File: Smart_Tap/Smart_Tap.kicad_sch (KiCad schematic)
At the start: 30 parts, among them IC1 TCRT5000L, IC2 TCRT5000L, IC3 PIC16C745-I_SO, J1 USB_B_Micro, J2 Conn_01x02_Female, J3 USB_B_Micro, M1 Motor_Servo, Q1 BC547, U1 MCP73831-2-OT, U2 LM393, U3 LM393, U4 DRV8833PW

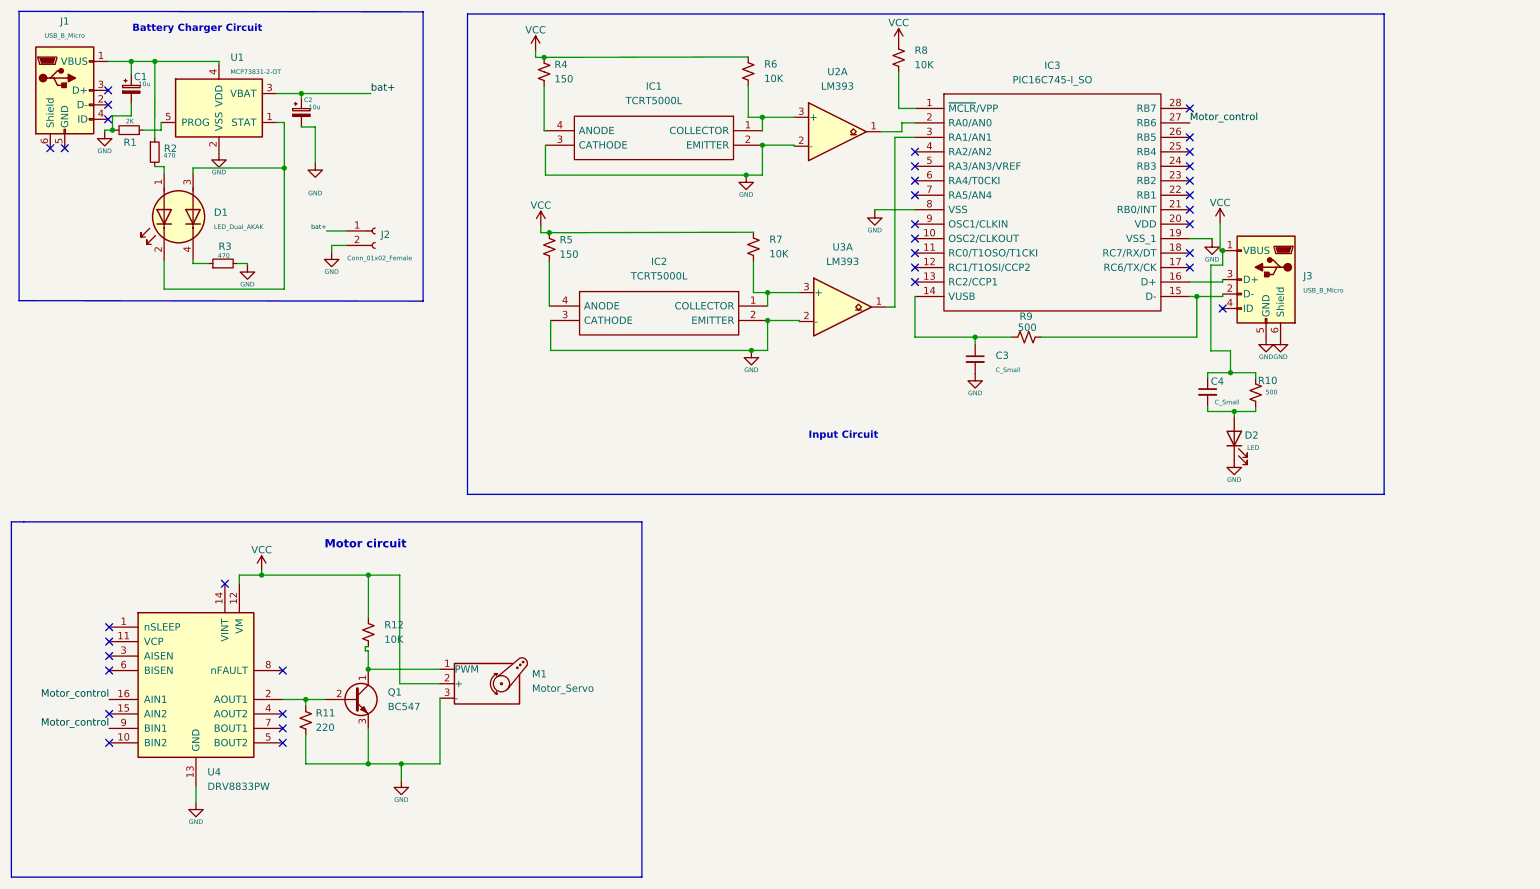
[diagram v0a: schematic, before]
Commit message: Updated Schematic
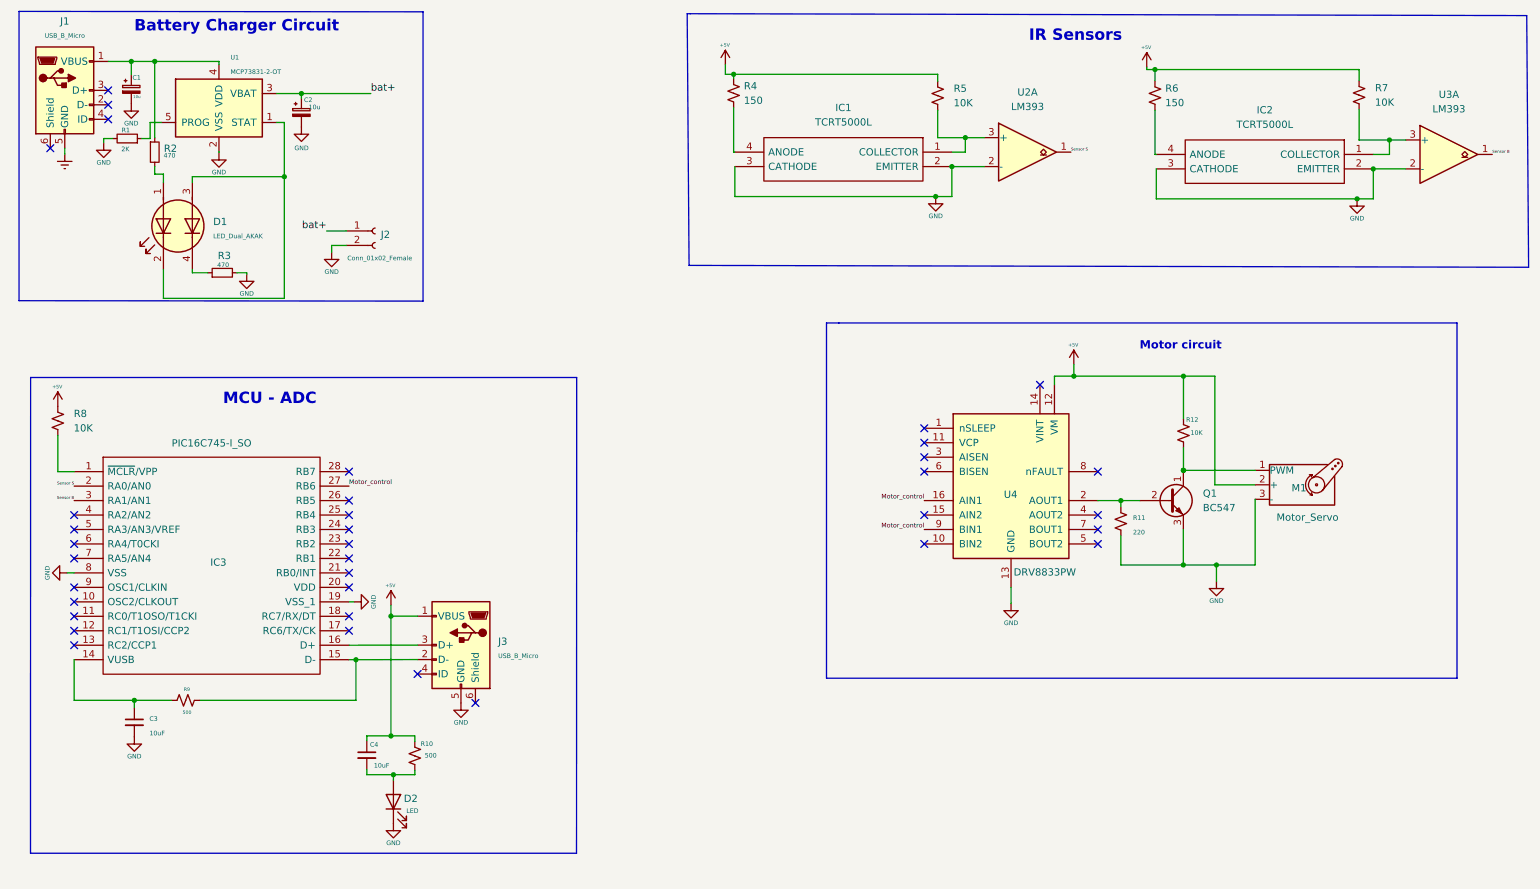
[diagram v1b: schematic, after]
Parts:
- C3, C4: value C_Small -> 10uF
- R5: value 150 -> 10K
- R6: value 10K -> 150
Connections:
- net GND: no longer J3.6 (Shield)
- net at R5.2: now also IC1.1 (COLLECTOR), U2.3 (+); no longer IC2.4 (ANODE)
- net Sensor B: now reaches IC3.3 (RA1/AN1), U3.1
- net Sensor S: now reaches IC3.2 (RA0/AN0), U2.1
- net Earth: now reaches J1.5 (GND)
- net VCC renamed +5V
- new net: IC2.4 (ANODE), R6.2
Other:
- note added: "IR Sensors"
- note added: "MCU - ADC"
- note removed: "Input Circuit"
- moved on the sheet: C3, C4, D1, D2, IC3, J3, M1, Q1, R1, R10, R11, R12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
